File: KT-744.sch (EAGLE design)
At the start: 41 parts, among them Q1 2T1, Q2 G1, Q3 G1, SW2 black

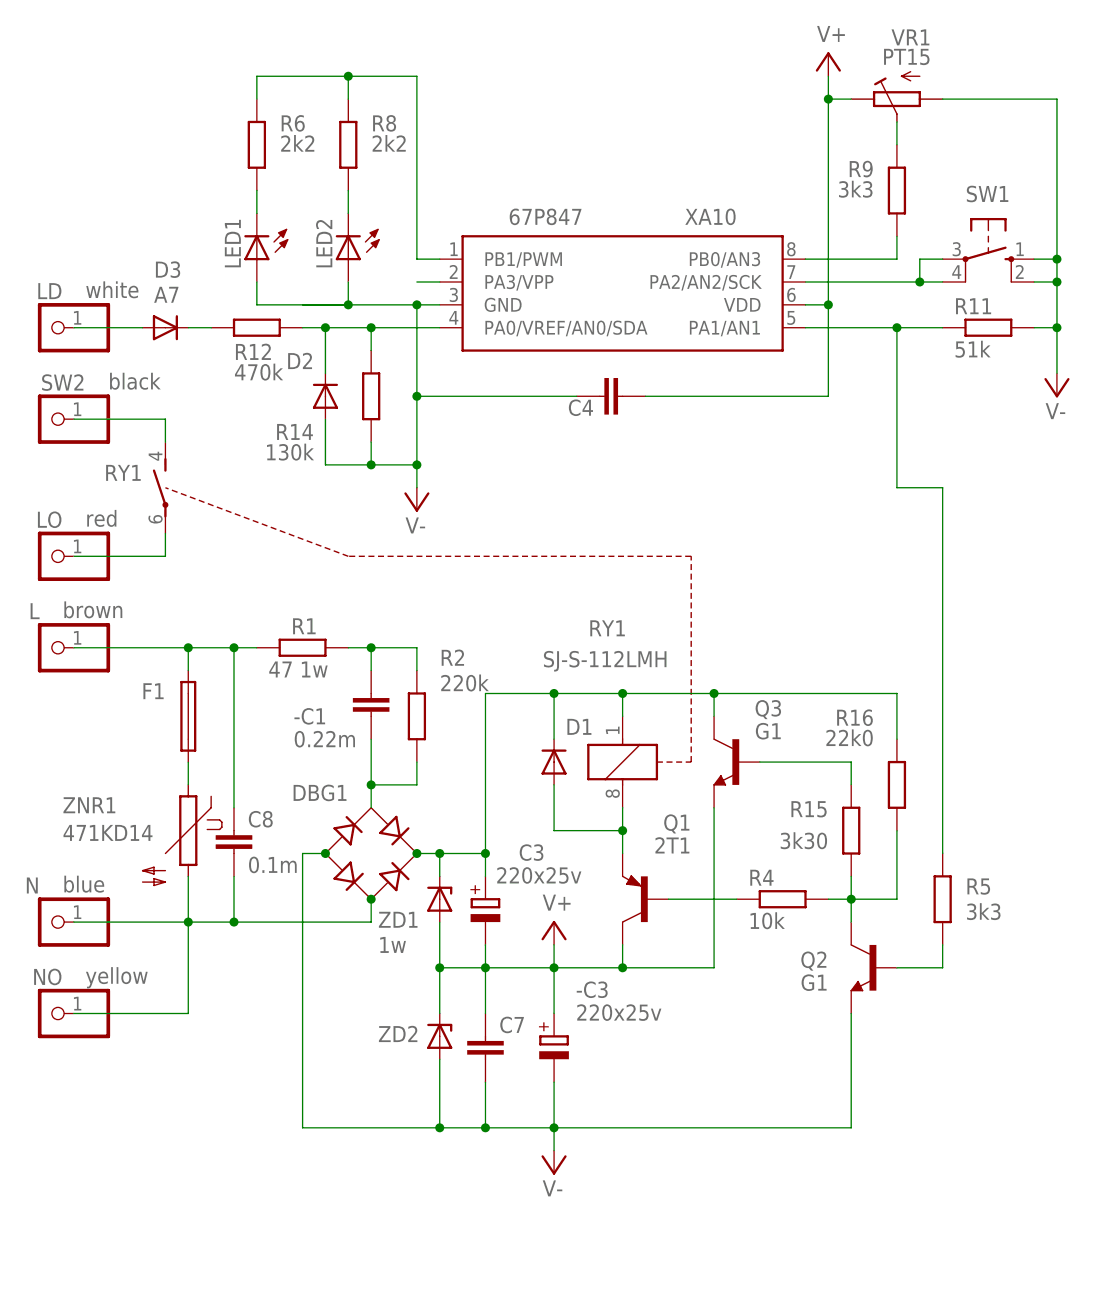
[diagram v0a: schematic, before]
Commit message: .
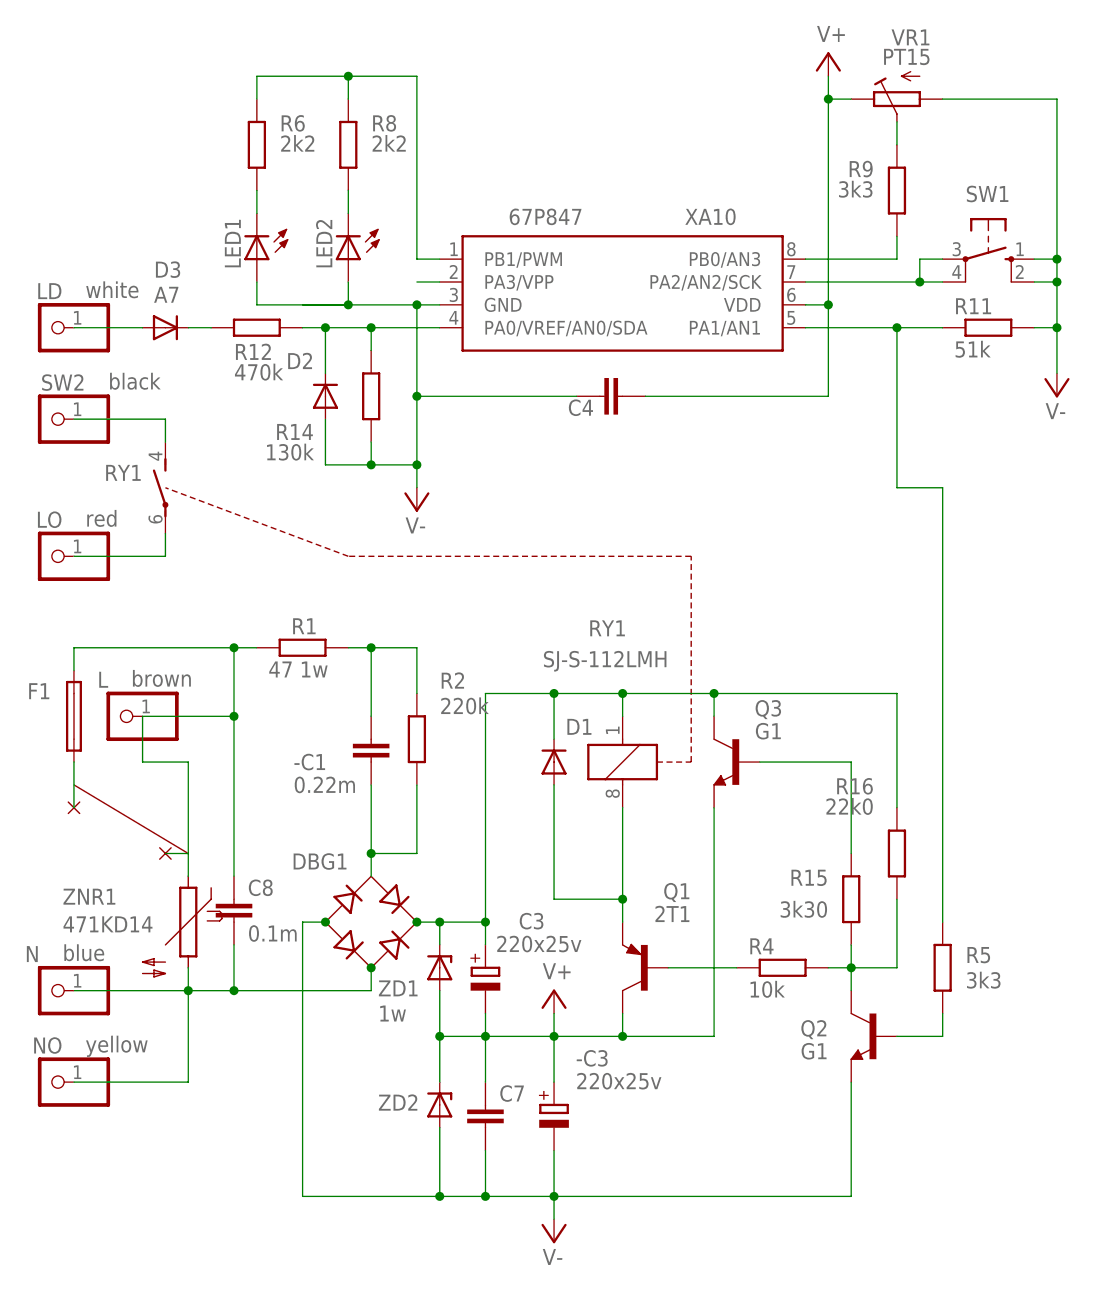
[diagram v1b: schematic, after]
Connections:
- removed net N$9: F1.1, ZNR1.1
- new net N$23: F1.1
- net N$4: now also ZNR1.1
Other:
- note added: "0 1 2 3 4 5 6 7 8 9 10 11 12 13 14 15 16 17 18 19 20 21 22 23 24 25 26 27 28 29 30 31 32 33 34 35 36"
- moved on the sheet: -C1, -C3, C3, C7, C8, DBG1, F1, L, N, NO, Q1, Q2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
